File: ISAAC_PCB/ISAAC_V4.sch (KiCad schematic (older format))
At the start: 53 parts, among them J1 Conn_02x04_Top_Bottom, J2 Conn_02x04_Top_Bottom, J3 Screw_Terminal_01x02, J4 XT60PW-M, U10 DMN4026SSD, U11 LM337_TO3, U2 DMN4026SSD, U3 DMN4026SSD, U4 DMN4026SSD, U5 DMN4026SSD, U6 module_mpu6050, U7 DMN4026SSD, U8 DMN4026SSD, U9 DMN4026SSD

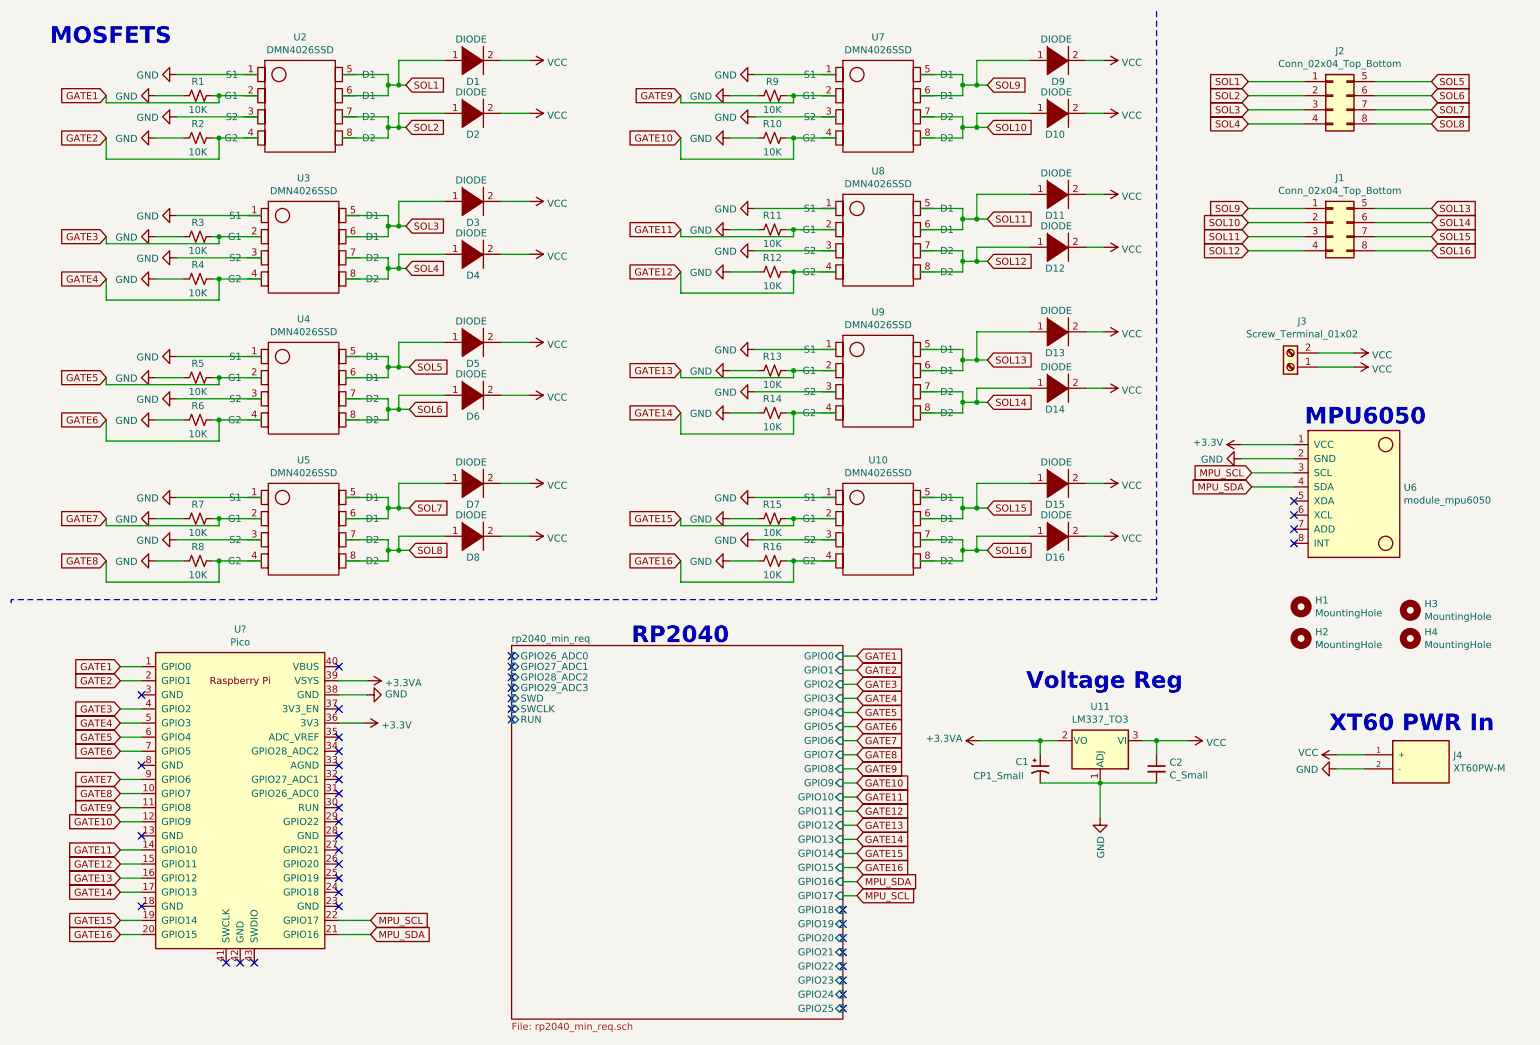
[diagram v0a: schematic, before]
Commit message: Updated Everything Again!
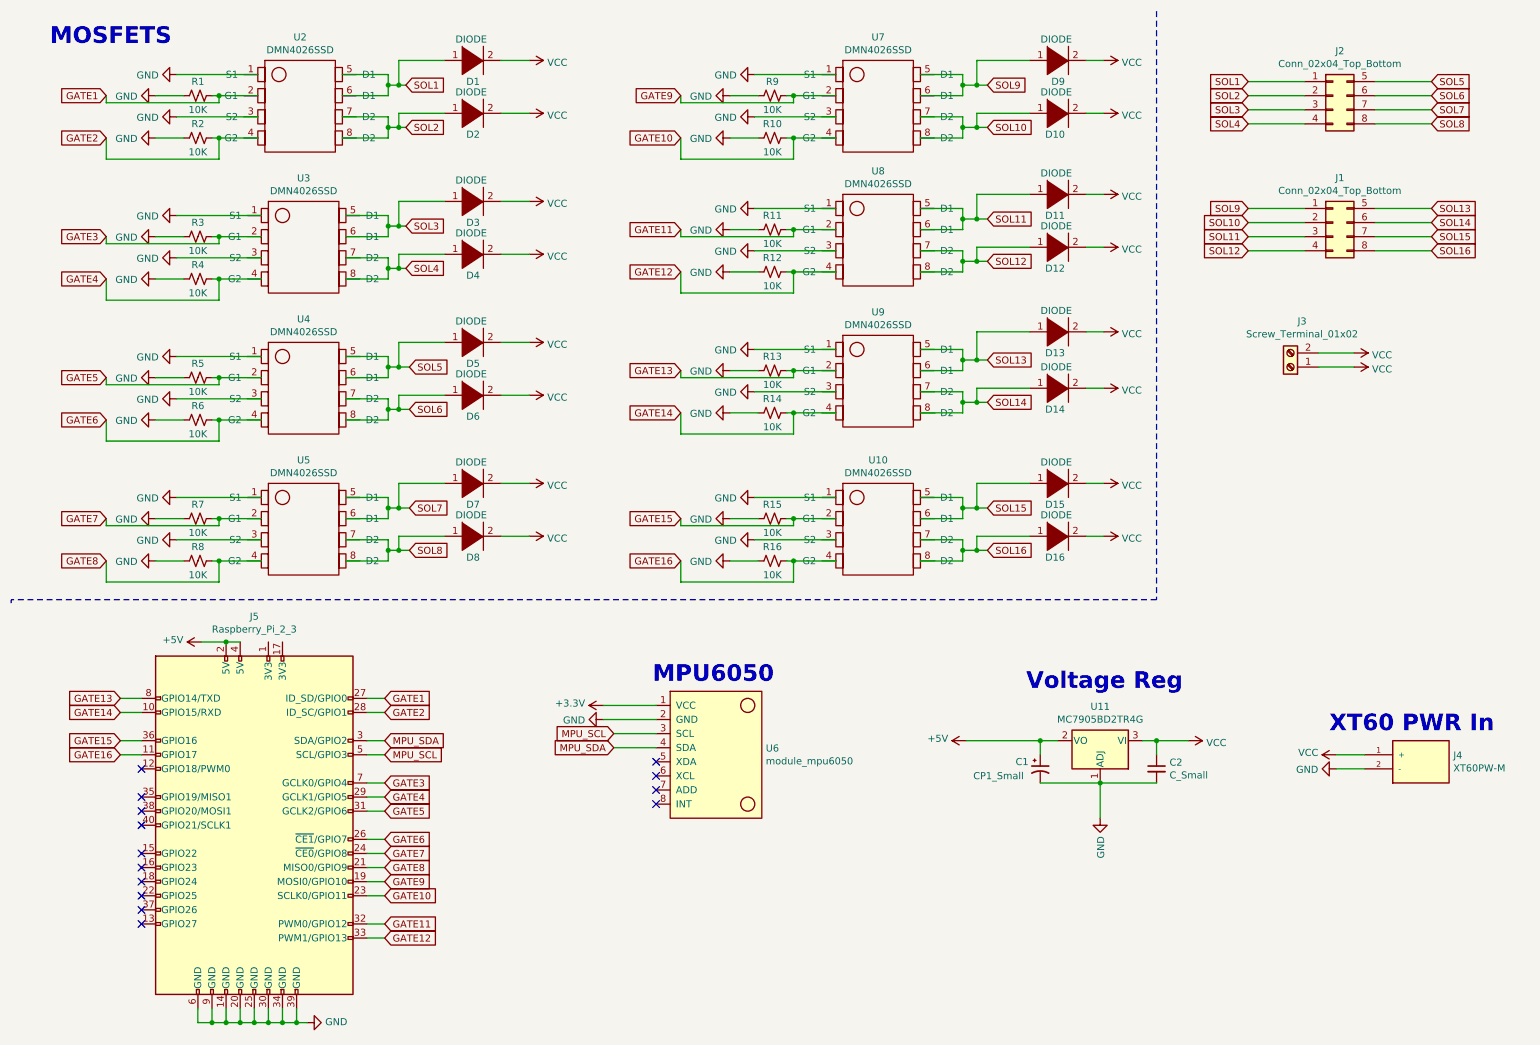
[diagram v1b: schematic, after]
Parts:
- removed H1, H2, H3, H4: MountingHole, MountingHole:MountingHole_3.2mm_M3, symbol Mechanical:MountingHole
- removed U?: Pico, RPi_Pico:RPi_Pico_SMD_TH, symbol MCU_RaspberryPi_and_Boards:Pico
- added J5: Raspberry_Pi_2_3, footprints:Pin_Header_Straight_2x20, symbol Connector:Raspberry_Pi_2_3
- U11: value LM337_TO3 -> MC7905BD2TR4G; footprint footprints:SOT230P696X180-4N -> footprints:TO254P1524X483-3
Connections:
- net GATE1: now also J5.27 (ID_SD/GPIO0)
- net GATE10: now also J5.23 (SCLK0/GPIO11)
- net GATE11: now also J5.32 (PWM0/GPIO12)
- net GATE12: now also J5.33 (PWM1/GPIO13)
- net GATE13: now also J5.8 (GPIO14/TXD)
- net GATE14: now also J5.10 (GPIO15/RXD)
- net GATE15: now also J5.36 (GPIO16)
- net GATE16: now also J5.11 (GPIO17)
- net GATE2: now also J5.28 (ID_SC/GPIO1)
- net GATE3: now also J5.7 (GCLK0/GPIO4)
- net GATE4: now also J5.29 (GCLK1/GPIO5)
- net GATE5: now also J5.31 (GCLK2/GPIO6)
- net GATE6: now also J5.26 (~CE1~/GPIO7)
- net GATE7: now also J5.24 (~CE0~/GPIO8)
- net GATE8: now also J5.21 (MISO0/GPIO9)
- net GATE9: now also J5.19 (MOSI0/GPIO10)
- net GND: now also J5.14 (GND), J5.20 (GND), J5.25 (GND), J5.30 (GND), J5.34 (GND), J5.39 (GND), J5.6 (GND), J5.9 (GND)
- net MPU_SCL: now also J5.5 (SCL/GPIO3)
- net MPU_SDA: now also J5.3 (SDA/GPIO2)
- net +3.3VA renamed +5V
- net +5V: now also J5.2 (5V), J5.4 (5V)
- no-connect marks 41 -> 14
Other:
- note removed: "RP2040\n"
- moved on the sheet: U6
